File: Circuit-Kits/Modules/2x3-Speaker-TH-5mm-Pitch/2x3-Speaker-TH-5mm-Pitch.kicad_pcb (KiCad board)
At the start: 2 copper layers, 23.5 x 15.6 mm, 1 part

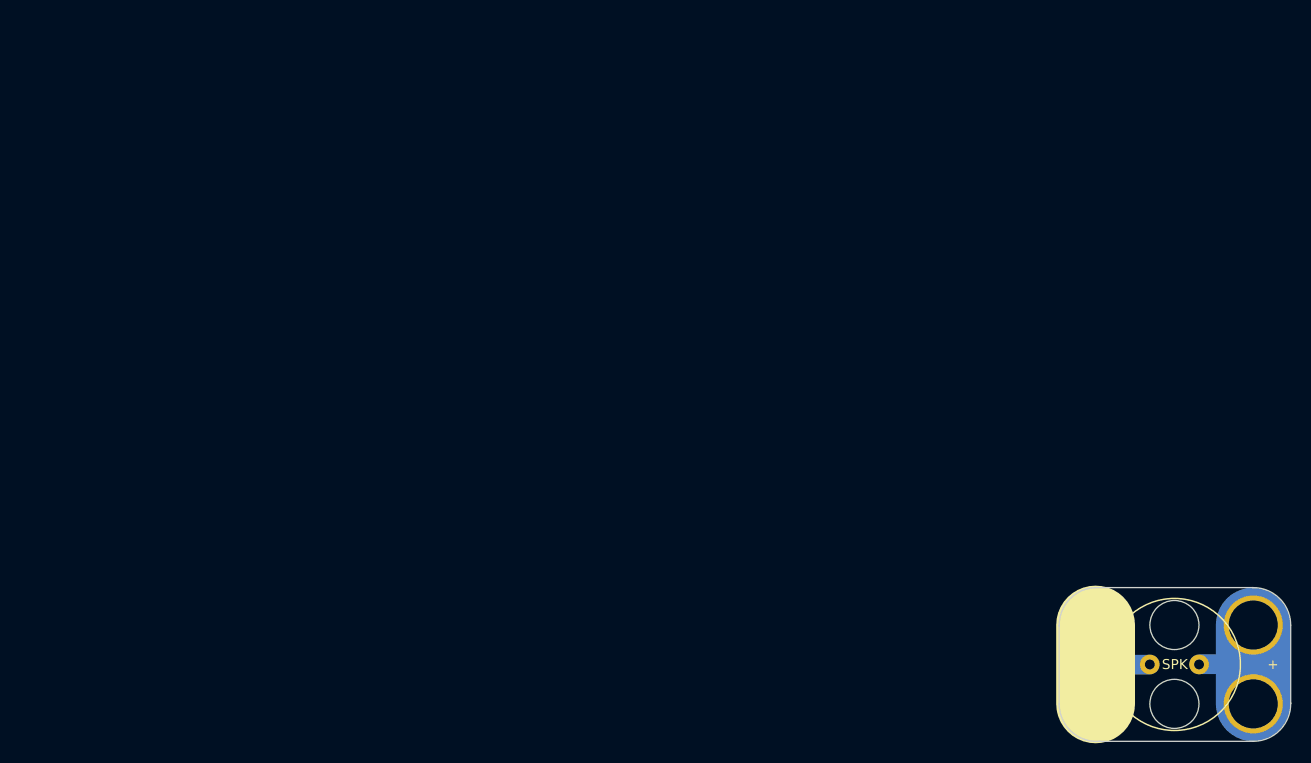
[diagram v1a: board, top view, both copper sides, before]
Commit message: Last of public release updates.
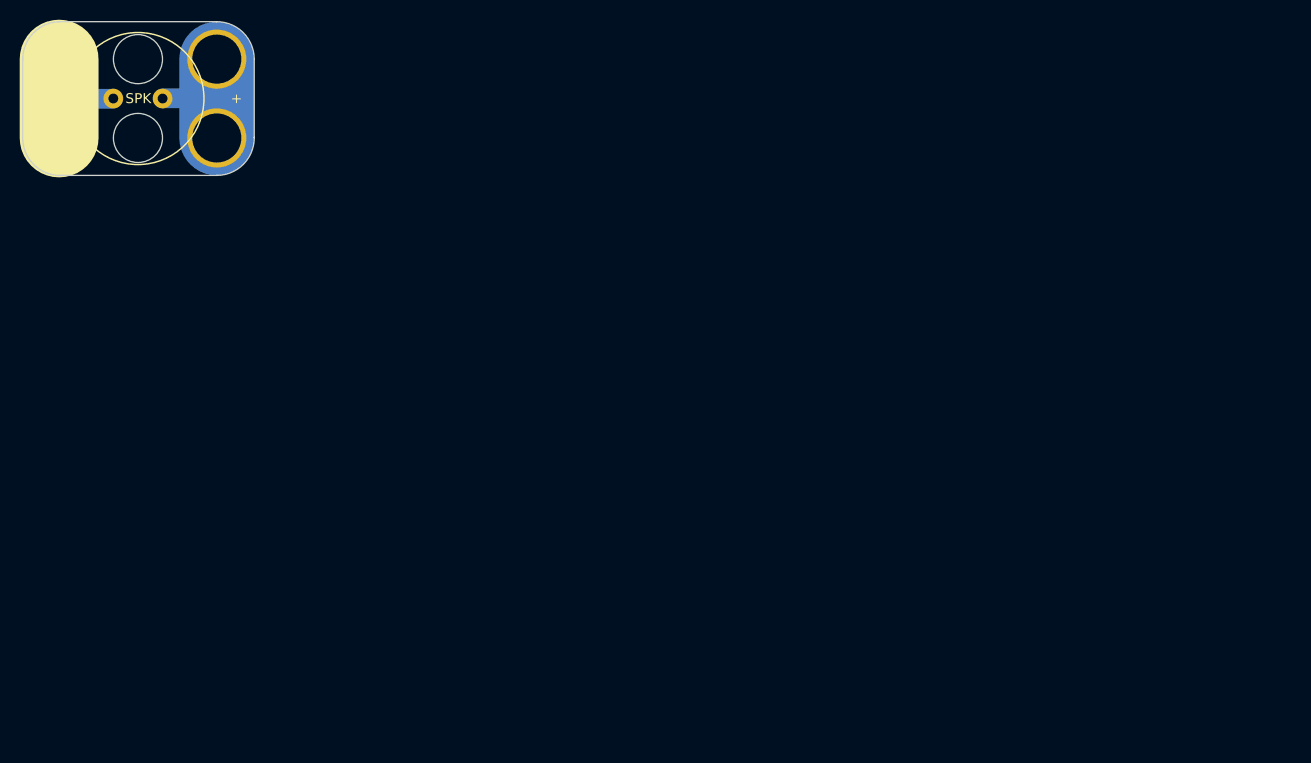
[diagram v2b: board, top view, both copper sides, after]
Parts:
- moved SPK1 119.8 mm to (24.9, 44.8)
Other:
- board text added: "FABRICATION NOTES 1. THIS IS A 2 LAYER BOARD. 2. EXTERNAL LAYERS SHALL HAVE 1 OZ COPPER. 3. MATERIAL: FR4 AND 0.062 INCH +/- 10% THICK. 4. BOARDS SHALL BE ROHS COMPLIANT. 5. MANUFACTURE IN ACCORDANCE WITH IPC-6012 CLASS 2 6. MASK: BOTH SIDES OF THE BOARD SHALL HAVE SOLDER MASK (BLACK) OVER BARE COPPER. 7. SILK: BOTH SIDES OF THE BOARD SHALL HAVE WHITE SILK. DO NOT PLACE SILK OVER BARE COPPER. 8. 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"
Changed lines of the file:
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@@
     (area 104.572999 74.854999 178.510001 123.265001)
     (thickness 1.6)
-    (drawings 18)
+    (drawings 2)
     (tracks 0)
     (zones 0)
@@
   )
   (module Crazy_Circuits:SPEAKER-PIEZO-5MMPitch-PS12-PS14-2x3 (layer F.Cu)
-    (at 130.05 102.235)
+    (at 24.8686 44.8056)
     (descr "piezo speaker 12 mm")
     (tags "buzzer speaker piezo")
@@
     (pad 2 thru_hole circle (at 10.5 -4) (size 2 2) (drill 1.00076) (layers *.Cu *.Mask)
       (net 2 /2))
-    (pad 1 thru_hole circle (at 0 0) (size 6 6) (drill 4.98) (layers *.Cu *.Mask)
+    (pad 1 thru_hole circle (at 0 0) (size 6 6) (drill 4.98) (layers *.Cu B.Mask)
       (net 1 /1))
-    (pad 2 thru_hole circle (at 16 0) (size 6 6) (drill 4.98) (layers *.Cu *.Mask)
+    (pad 2 thru_hole circle (at 16 0) (size 6 6) (drill 4.98) (layers *.Cu B.Mask)
       (net 2 /2))
-    (pad 2 thru_hole circle (at 16 -8) (size 6 6) (drill 4.98) (layers *.Cu *.Mask)
+    (pad 2 thru_hole circle (at 16 -8) (size 6 6) (drill 4.98) (layers *.Cu B.Mask)
       (net 2 /2))
-    (pad 1 thru_hole circle (at 0 -8) (size 6 6) (drill 4.98) (layers *.Cu *.Mask)
+    (pad 1 thru_hole circle (at 0 -8) (size 6 6) (drill 4.98) (layers *.Cu B.Mask)
       (net 1 /1))
     (pad "" np_thru_hole circle (at 8 -8) (size 4.98 4.98) (drill 4.98) (layers *.Cu))
     (pad "" np_thru_hole circle (at 8 0) (size 4.98 4.98) (drill 4.98) (layers *.Cu))
   )
-  (gr_text SPK (at 138.08964 98.23196) (layer F.SilkS)
+  (gr_text "FABRICATION NOTES\n\n1. THIS IS A 2 LAYER BOARD. \n2. EXTERNAL LAYERS SHALL HAVE 1 OZ COPPER.\n3. MATERIAL: FR4 AND 0.062 INCH +/- 10% THICK.\n4. BOARDS SHALL BE ROHS COMPLIANT. \n5. MANUFACTURE IN ACCORDANCE WITH IPC-6012 CLASS 2\n6. MASK: BOTH SIDES OF THE BOARD SHALL HAVE \n   SOLDER MASK (BLACK) OVER BARE COPPER. \n7. SILK: BOTH SIDES OF THE BOARD SHALL HAVE WHITE SILK. \n   DO NOT PLACE SILK OVER BARE COPPER.\n8. FINISH: ENIG.\n9. MINIMUM TRACE WIDTH - 0.006 INCH.\n   MINIMUM SPACE - 0.006 INCH.\n   MINIMUM HOLE DIA - 0.013 INCH. \n10. MAX HOLE PLACEMENT TOLERANCE OF +/- 0.003 INCH.\n11. MAX HOLE DIAMETER TOLERANCE OF +/- 0.003 INCH AFTER PLATING." (at 6.6802 94.4118) (layer Dwgs.User)
+    (effects (font (size 2.54 2.54) (thickness 0.254)) (justify left))
+  )
+  (gr_text SPK (at 32.90824 40.80256) (layer F.SilkS)
     (effects (font (size 1.016 1.016) (thickness 0.1524)))
   )
-  (gr_circle (center 117.348 76.962) (end 118.618 76.962) (layer Dwgs.User) (width 0.15))
-  (gr_line (start 114.427 78.994) (end 114.427 74.93) (angle 90) (layer Dwgs.User) (width 0.15))
-  (gr_line (start 120.269 78.994) (end 114.427 78.994) (angle 90) (layer Dwgs.User) (width 0.15))
-  (gr_line (start 120.269 74.93) (end 120.269 78.994) (angle 90) (layer Dwgs.User) (width 0.15))
-  (gr_line (start 114.427 74.93) (end 120.269 74.93) (angle 90) (layer Dwgs.User) (width 0.15))
-  (gr_line (start 120.523 93.98) (end 104.648 93.98) (angle 90) (layer Dwgs.User) (width 0.15))
-  (gr_line (start 173.355 102.235) (end 173.355 94.615) (angle 90) (layer Dwgs.User) (width 0.15))
-  (gr_line (start 178.435 102.235) (end 173.355 102.235) (angle 90) (layer Dwgs.User) (width 0.15))
-  (gr_line (start 178.435 94.615) (end 178.435 102.235) (angle 90) (layer Dwgs.User) (width 0.15))
-  (gr_line (start 173.355 94.615) (end 178.435 94.615) (angle 90) (layer Dwgs.User) (width 0.15))
-  (gr_line (start 109.093 123.19) (end 109.093 114.3) (angle 90) (layer Dwgs.User) (width 0.15))
-  (gr_line (start 122.428 123.19) (end 109.093 123.19) (angle 90) (layer Dwgs.User) (width 0.15))
-  (gr_line (start 122.428 114.3) (end 122.428 123.19) (angle 90) (layer Dwgs.User) (width 0.15))
-  (gr_line (start 109.093 114.3) (end 122.428 114.3) (angle 90) (layer Dwgs.User) (width 0.15))
-  (gr_line (start 104.648 93.98) (end 104.648 82.55) (angle 90) (layer Dwgs.User) (width 0.15))
-  (gr_line (start 120.523 82.55) (end 120.523 93.98) (angle 90) (layer Dwgs.User) (width 0.15))
-  (gr_line (start 104.648 82.55) (end 120.523 82.55) (angle 90) (layer Dwgs.User) (width 0.15))
 )
